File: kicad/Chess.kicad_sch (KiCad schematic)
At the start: 71 parts, among them J2 Conn_01x08_Pin, U1 CD74HC4067M, U12 A1302xUA, U13 A1302xUA, U14 A1302xUA, U15 A1302xUA, U16 A1302xUA, U17 A1302xUA, U18 A1302xUA, U19 A1302xUA, U2 ADS1015IDGS, U20 A1302xUA, U21 A1302xUA, U22 A1302xUA, U23 A1302xUA, U24 A1302xUA, U25 A1302xUA, U26 A1302xUA, U27 A1302xUA, U28 A1302xUA, U29 A1302xUA, U3 MP1584EN, U30 A1302xUA, U31 A1302xUA, U32 A1302xUA, U33 A1302xUA, U34 A1302xUA, U35 A1302xUA, U36 A1302xUA, U37 A1302xUA, U38 A1302xUA, U39 A1302xUA, U4 CD74HC4067M, U40 A1302xUA, U41 A1302xUA, U42 A1302xUA, U43 A1302xUA, U44 A1302xUA, U45 A1302xUA, U46 A1302xUA, U47 A1302xUA, U48 A1302xUA, U49 A1302xUA, U5 CD74HC4067M, U50 A1302xUA, U51 A1302xUA, U52 A1302xUA, U53 A1302xUA, U54 A1302xUA, U55 A1302xUA, U56 A1302xUA, U57 A1302xUA, U58 A1302xUA, U59 A1302xUA, U6 CD74HC4067M, U60 A1302xUA, U61 A1302xUA, U62 A1302xUA, U63 A1302xUA, U64 A1302xUA, U65 A1302xUA, U66 A1302xUA, U67 A1302xUA, U68 A1302xUA, U69 A1302xUA, U70 A1302xUA, U71 A1302xUA, U72 A1302xUA, U73 A1302xUA, U74 A1302xUA, U75 A1302xUA

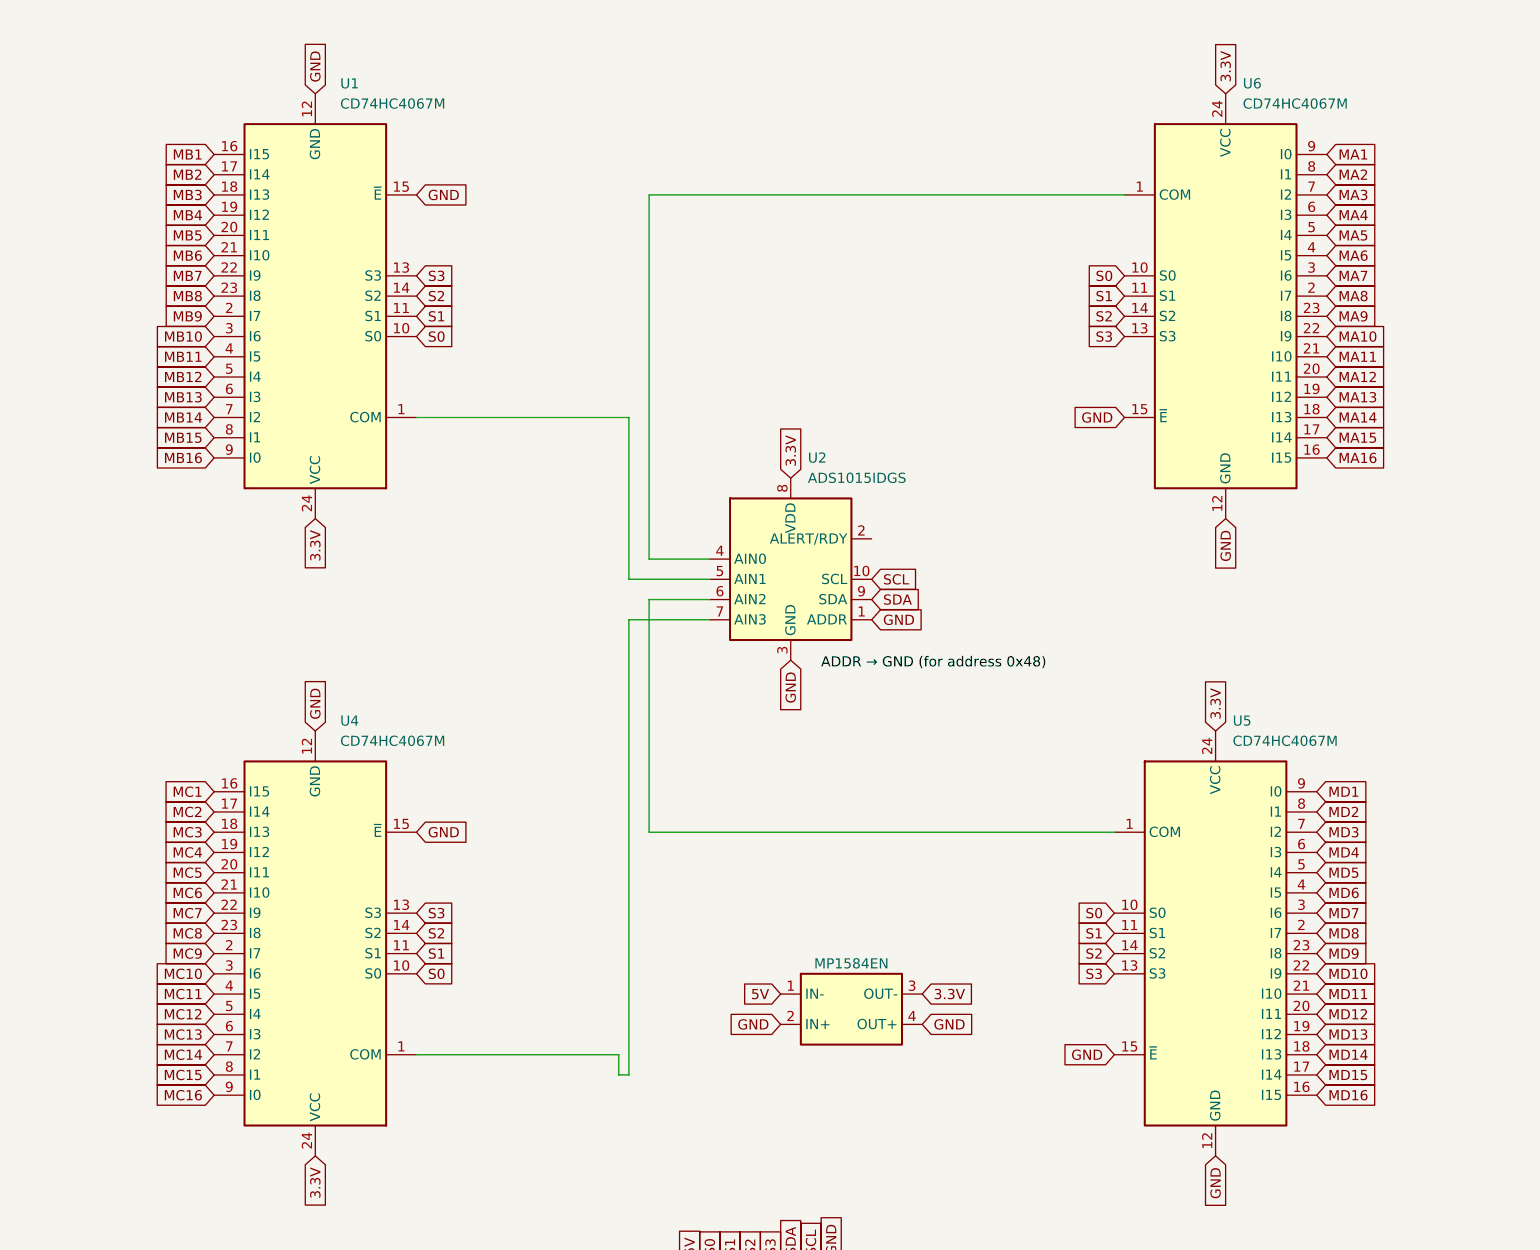
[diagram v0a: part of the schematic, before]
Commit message: routing v2
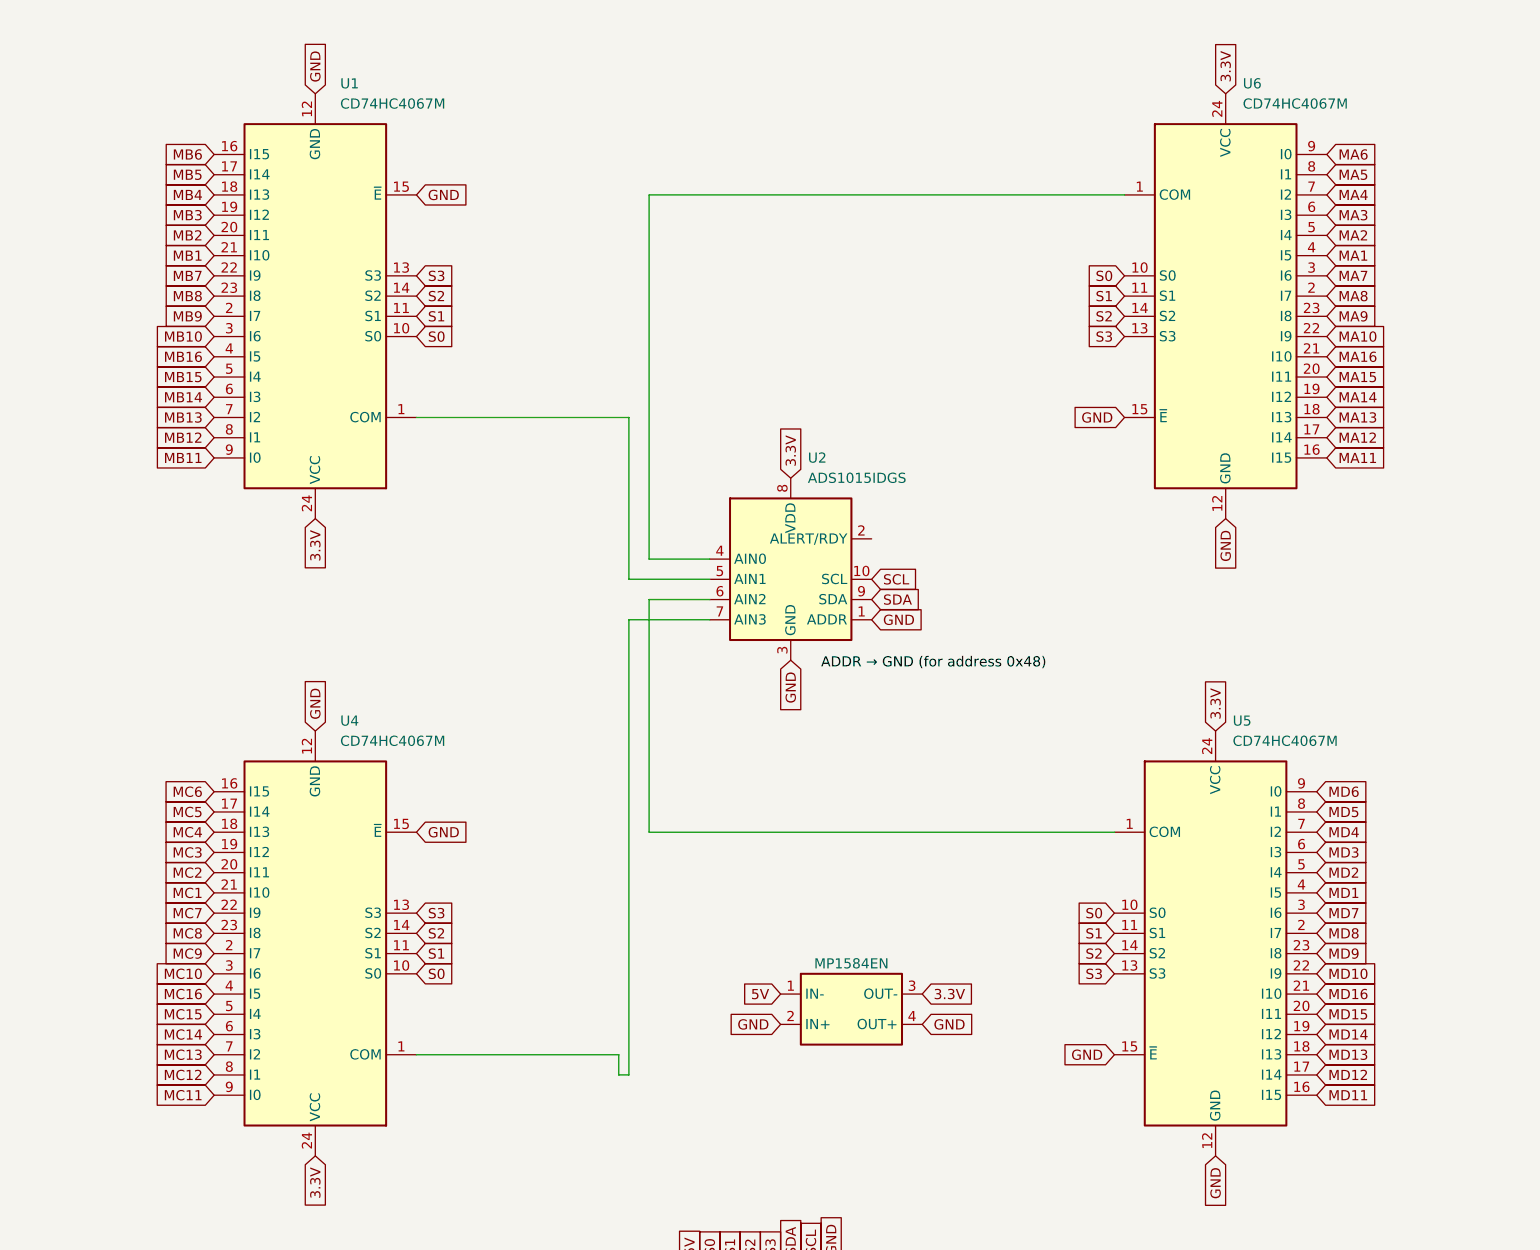
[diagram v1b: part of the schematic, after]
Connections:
- net MA1: now also U6.4 (I5); no longer U6.9 (I0)
- net MA11: now also U6.16 (I15); no longer U6.21 (I10)
- net MA12: now also U6.17 (I14); no longer U6.20 (I11)
- net MA13: now also U6.18 (I13); no longer U6.19 (I12)
- net MA14: now also U6.19 (I12); no longer U6.18 (I13)
- net MA15: now also U6.20 (I11); no longer U6.17 (I14)
- net MA16: now also U6.21 (I10); no longer U6.16 (I15)
- net MA2: now also U6.5 (I4); no longer U6.8 (I1)
- net MA3: now also U6.6 (I3); no longer U6.7 (I2)
- net MA4: now also U6.7 (I2); no longer U6.6 (I3)
- net MA5: now also U6.8 (I1); no longer U6.5 (I4)
- net MA6: now also U6.9 (I0); no longer U6.4 (I5)
- net MB1: now also U1.21 (I10); no longer U1.16 (I15)
- net MB11: now also U1.9 (I0); no longer U1.4 (I5)
- net MB12: now also U1.8 (I1); no longer U1.5 (I4)
- net MB13: now also U1.7 (I2); no longer U1.6 (I3)
- net MB14: now also U1.6 (I3); no longer U1.7 (I2)
- net MB15: now also U1.5 (I4); no longer U1.8 (I1)
- net MB16: now also U1.4 (I5); no longer U1.9 (I0)
- net MB2: now also U1.20 (I11); no longer U1.17 (I14)
- net MB3: now also U1.19 (I12); no longer U1.18 (I13)
- net MB4: now also U1.18 (I13); no longer U1.19 (I12)
- net MB5: now also U1.17 (I14); no longer U1.20 (I11)
- net MB6: now also U1.16 (I15); no longer U1.21 (I10)
- net MC1: now also U4.21 (I10); no longer U4.16 (I15)
- net MC11: now also U4.9 (I0); no longer U4.4 (I5)
- net MC12: now also U4.8 (I1); no longer U4.5 (I4)
- net MC13: now also U4.7 (I2); no longer U4.6 (I3)
- net MC14: now also U4.6 (I3); no longer U4.7 (I2)
- net MC15: now also U4.5 (I4); no longer U4.8 (I1)
- net MC16: now also U4.4 (I5); no longer U4.9 (I0)
- net MC2: now also U4.20 (I11); no longer U4.17 (I14)
- net MC3: now also U4.19 (I12); no longer U4.18 (I13)
- net MC4: now also U4.18 (I13); no longer U4.19 (I12)
- net MC5: now also U4.17 (I14); no longer U4.20 (I11)
- net MC6: now also U4.16 (I15); no longer U4.21 (I10)
- net MD1: now also U5.4 (I5); no longer U5.9 (I0)
- net MD11: now also U5.16 (I15); no longer U5.21 (I10)
- net MD12: now also U5.17 (I14); no longer U5.20 (I11)
- net MD13: now also U5.18 (I13); no longer U5.19 (I12)
- net MD14: now also U5.19 (I12); no longer U5.18 (I13)
- net MD15: now also U5.20 (I11); no longer U5.17 (I14)
- net MD16: now also U5.21 (I10); no longer U5.16 (I15)
- net MD2: now also U5.5 (I4); no longer U5.8 (I1)
- net MD3: now also U5.6 (I3); no longer U5.7 (I2)
- net MD4: now also U5.7 (I2); no longer U5.6 (I3)
- net MD5: now also U5.8 (I1); no longer U5.5 (I4)
- net MD6: now also U5.9 (I0); no longer U5.4 (I5)
